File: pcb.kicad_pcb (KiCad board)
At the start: 2 copper layers, 95.1 x 95.1 mm, 186 parts, among them IC1 BQ25302RTER, IC2 SPV1040T, IC3 SI3483DDV-T1-BE3, IC4 SPV1040T, IC5 SPV1040T, J1 PTHF-126-02-GF-Q-368, J2 Sol_X+_X-, J3 Sol_Y+_Y-, J4 USB_B_Micro, J5 SWD, J6 Sol_Z+_Z-, Q1 NPN, Q2 NPN, Q3 NPN, Q4 NPN, Q5 NPN, SW1 SW_SPDT, U1 STM32F405RGT6, U2 LTC2990, U3 LTC2990, U4 LTC2990, Y1 16MHz

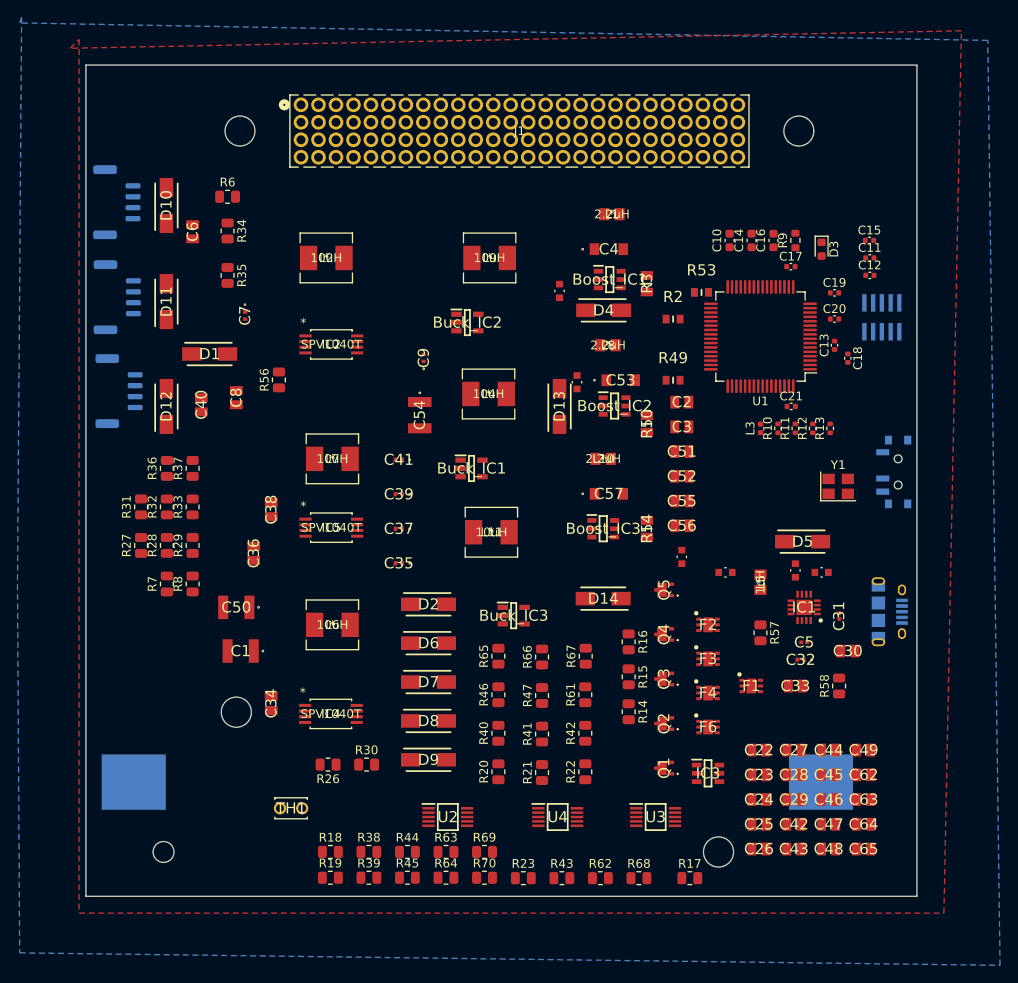
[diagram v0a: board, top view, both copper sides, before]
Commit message: updates
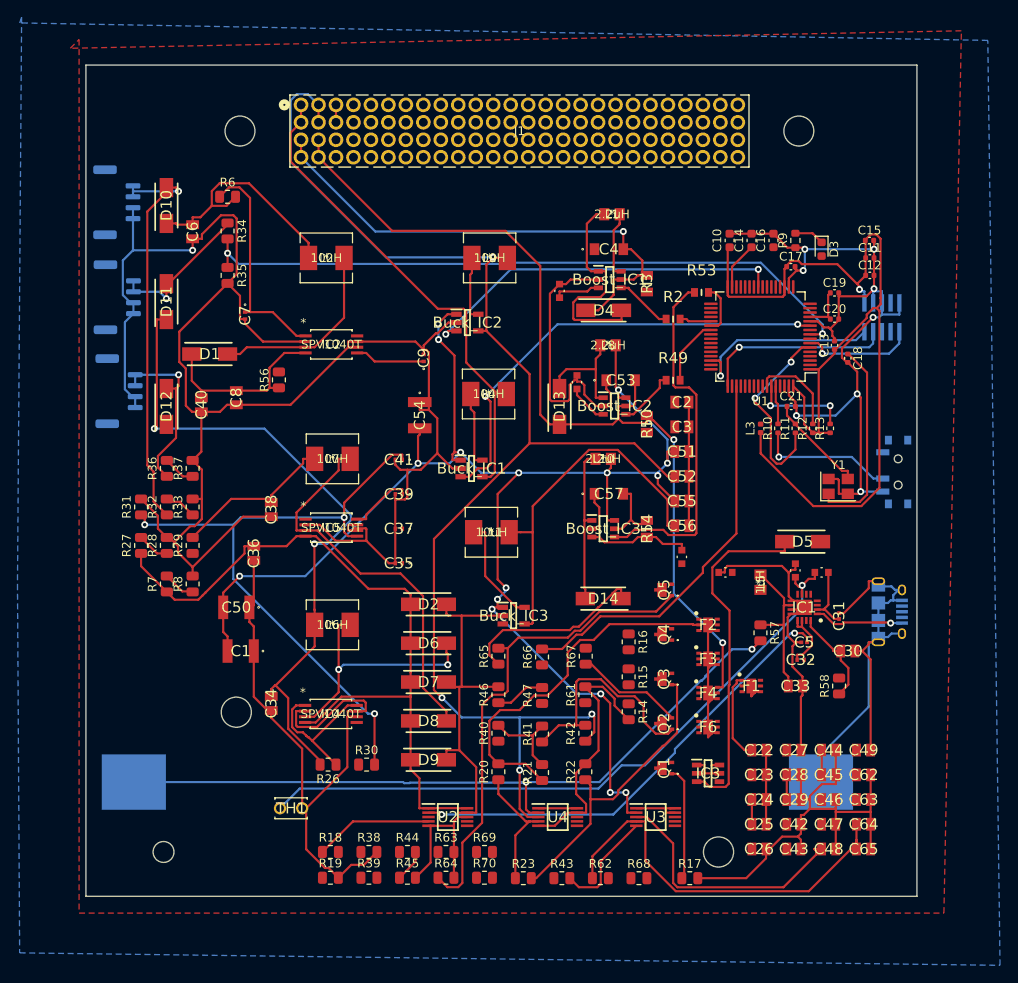
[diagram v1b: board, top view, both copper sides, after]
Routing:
- net Earth: track 0.00 -> 628.9 mm, vias 0 -> 1
- net +Vpp: track 0.00 -> 182.2 mm, vias 0 -> 16
- net 3.3V_ADCS: track 0.00 -> 156.9 mm, vias 0 -> 4
- net 5V_PAYLOAD: track 0.00 -> 134.7 mm, vias 0 -> 2
- net +3V3: track 0.00 -> 110.3 mm, vias 0 -> 1
- net MPPT_I+: track 0.00 -> 105.4 mm
- net GND: track 0.00 -> 93.8 mm, vias 0 -> 8
- net BAT_I-: track 0.00 -> 83.3 mm, vias 0 -> 2
- net SOL_Y_ADC: track 0.00 -> 77.4 mm, vias 0 -> 2
- net Net-(IC1-TS): track 0.00 -> 77.0 mm, vias 0 -> 1
- net Net-(D11-K): track 0.00 -> 76.9 mm, vias 0 -> 2
- net 5V_COMM: track 0.00 -> 76.0 mm
- net Net-(IC5-VCTRL): track 0.00 -> 73.6 mm, vias 0 -> 3
- net MPPT_I-: track 0.00 -> 63.3 mm, vias 0 -> 3
- net 3.3V_COMM: track 0.00 -> 59.7 mm
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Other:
- copper layers 2 -> 4
